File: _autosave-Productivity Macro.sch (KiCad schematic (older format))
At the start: 34 parts, among them SW1 SW_Push, SW2 Rotary_Encoder_Switch, SW3 Rotary_Encoder_Switch, U1 ATmega32U4-AU, Y1 16Mhz

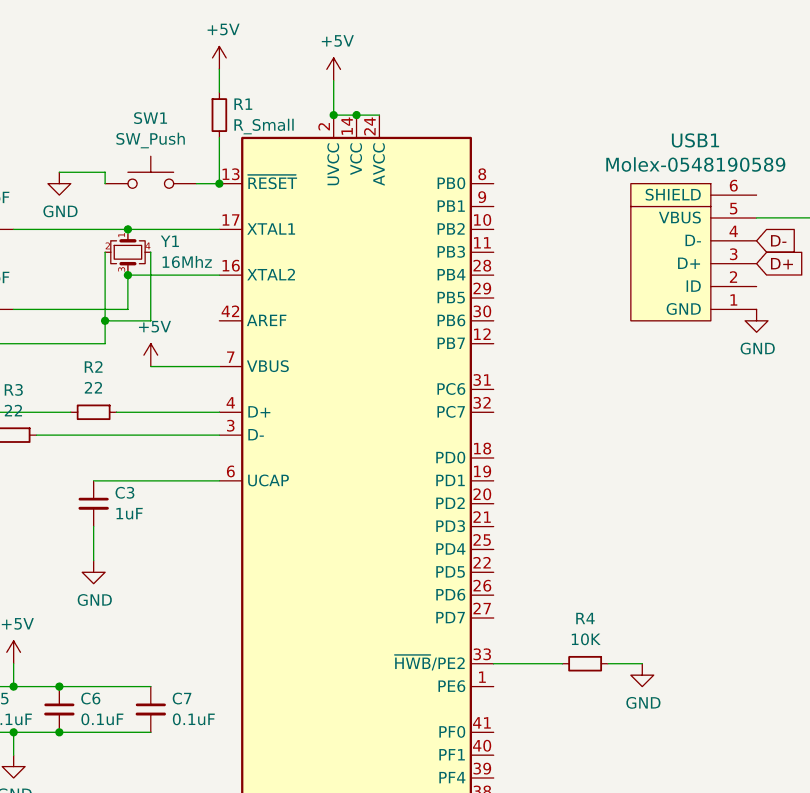
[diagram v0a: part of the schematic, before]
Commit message: process
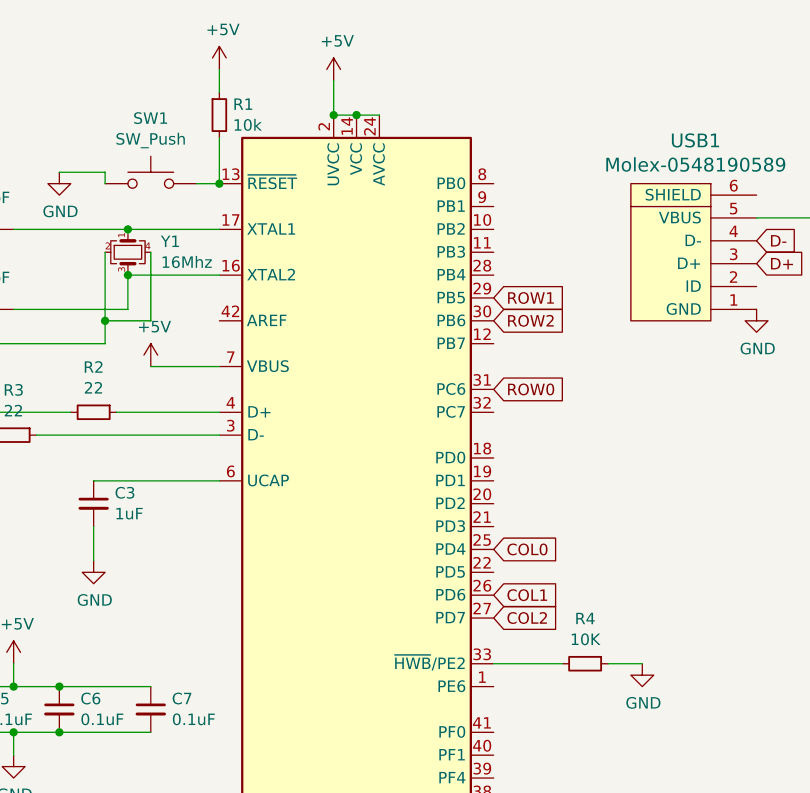
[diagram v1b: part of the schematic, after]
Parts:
- R1: value R_Small -> 10k
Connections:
- net COL0: now also U1.25 (PD4)
- net COL1: now also U1.26 (PD6)
- net COL2: now also U1.27 (PD7)
- net ROW0: now also U1.31 (PC6)
- net ROW1: now also U1.29 (PB5)
- net ROW2: now also U1.30 (PB6)
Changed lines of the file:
@@
 P 3700 1100
 F 0 "R1" H 3759 1146 50  0000 L CNN
-F 1 "R_Small" H 3759 1055 50  0000 L CNN
+F 1 "10k" H 3759 1055 50  0000 L CNN
 F 2 "Resistor_SMD:R_0805_2012Metric" H 3700 1100 50  0001 C CNN
 F 3 "~" H 3700 1100 50  0001 C CNN
@@
 	0    -1   -1   0
 $EndComp
+Text GLabel 4900 3000 2    50   Input ~ 0
+COL0
+Text GLabel 4900 2300 2    50   Input ~ 0
+ROW0
+Text GLabel 4900 1900 2    50   Input ~ 0
+ROW1
+Text GLabel 4900 3200 2    50   Input ~ 0
+COL1
+Text GLabel 4900 3300 2    50   Input ~ 0
+COL2
+Text GLabel 4900 2000 2    50   Input ~ 0
+ROW2
 $EndSCHEMATC

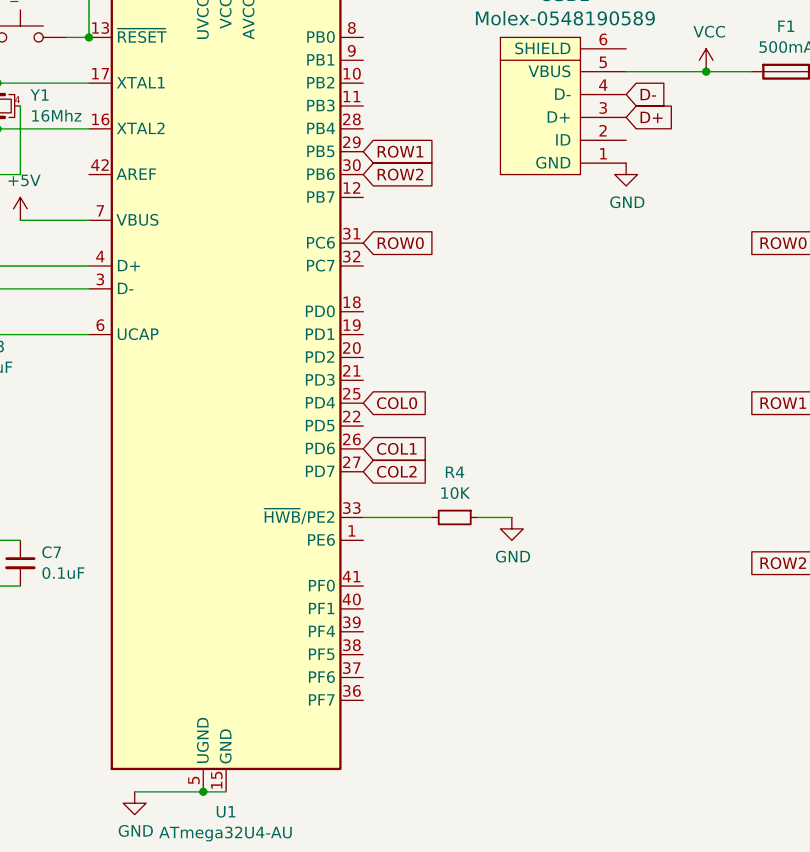
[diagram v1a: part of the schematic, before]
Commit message: this is stupid
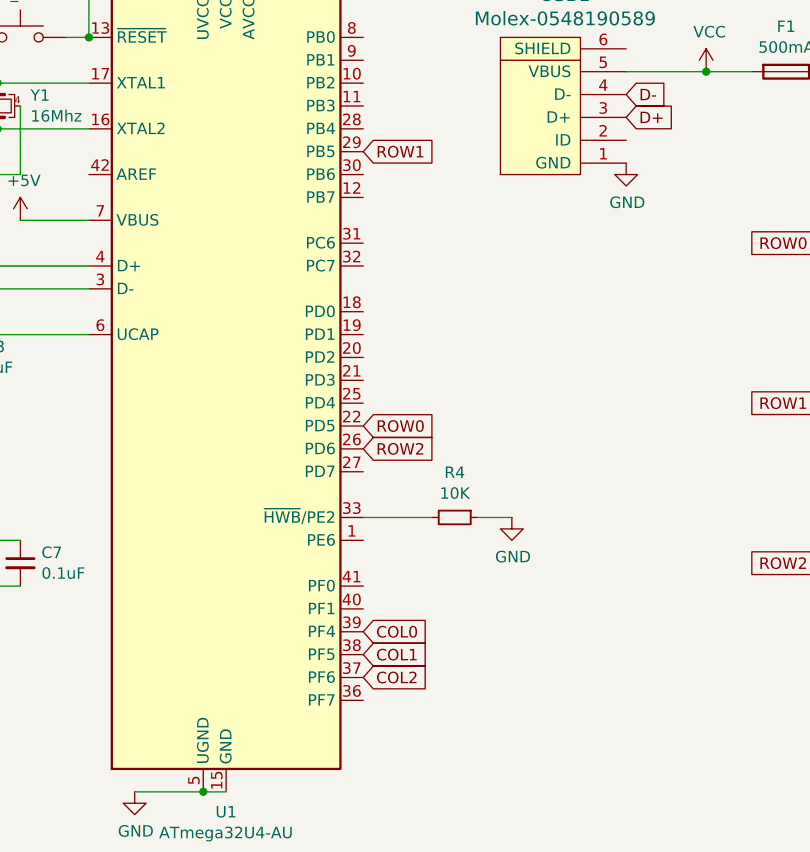
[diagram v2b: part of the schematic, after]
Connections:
- net COL0: now also U1.39 (PF4); no longer U1.25 (PD4)
- net COL1: now also U1.38 (PF5); no longer U1.26 (PD6)
- net COL2: now also U1.37 (PF6); no longer U1.27 (PD7)
- net ROW0: now also U1.22 (PD5); no longer U1.31 (PC6)
- net ROW2: now also U1.26 (PD6); no longer U1.30 (PB6)
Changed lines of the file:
@@
 	0    -1   -1   0
 $EndComp
-Text GLabel 4900 3000 2    50   Input ~ 0
+Text GLabel 4900 4000 2    50   Input ~ 0
 COL0
-Text GLabel 4900 2300 2    50   Input ~ 0
+Text GLabel 4900 3100 2    50   Input ~ 0
 ROW0
 Text GLabel 4900 1900 2    50   Input ~ 0
 ROW1
+Text GLabel 4900 4100 2    50   Input ~ 0
+COL1
+Text GLabel 4900 4200 2    50   Input ~ 0
+COL2
 Text GLabel 4900 3200 2    50   Input ~ 0
-COL1
-Text GLabel 4900 3300 2    50   Input ~ 0
-COL2
-Text GLabel 4900 2000 2    50   Input ~ 0
 ROW2
 $EndSCHEMATC
